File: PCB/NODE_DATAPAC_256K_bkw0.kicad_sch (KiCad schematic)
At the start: 28 parts, among them J1 Conn_02x20_Odd_Even, U1 74161, U10 62256, U2 74161, U3 74161, U4 74138, U5 74138, U6 74374, U7 62256, U8 62256, U9 62256

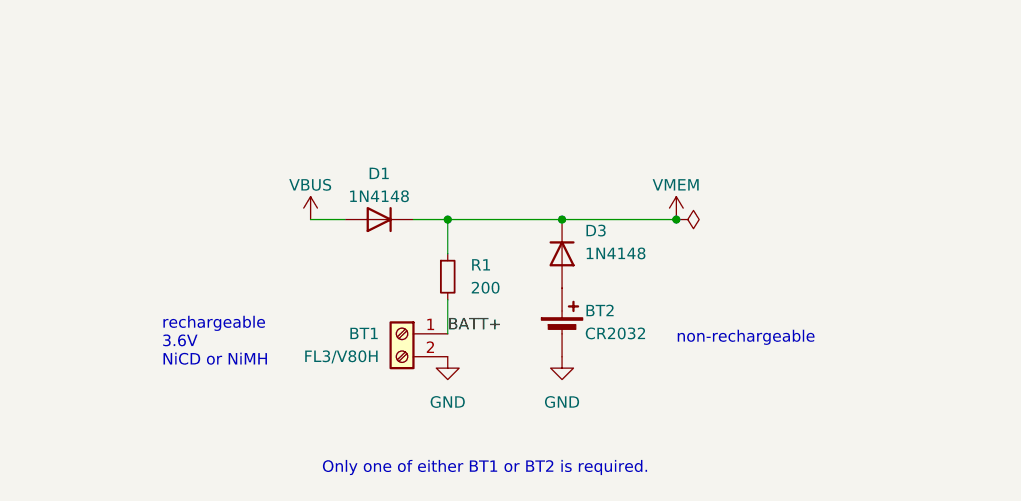
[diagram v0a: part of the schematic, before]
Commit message: readme, software, remove nimh from new board
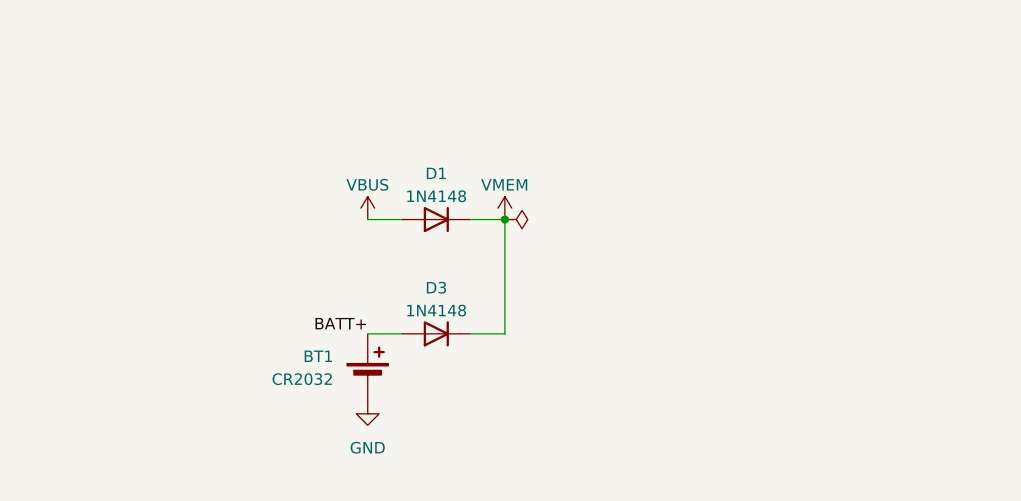
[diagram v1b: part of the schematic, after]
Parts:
- removed BT1: FL3/V80H, 000_LOCAL:CONN2_1776275-2, symbol 000_LOCAL:Screw_Terminal_01x02
- removed R1: 200, 000_LOCAL:R_Axial_DIN0207_L6.3mm_D2.5mm_P10.16mm_Horizontal, symbol 000_LOCAL:R
- U10, U7, U8, U9: symbol 000_LOCAL:62256-DIP -> 000_LOCAL:62256
- renumbered BT2 to BT1
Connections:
- net BATT+: now also BT1.1 (+), D3.2 (A)
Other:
- note removed: "Only one of either BT1 or BT2 is required."
- note removed: "non-rechargeable"
- note removed: "rechargeable 3.6V NiCD or NiMH"
- moved on the sheet: BT1, D1, D3
